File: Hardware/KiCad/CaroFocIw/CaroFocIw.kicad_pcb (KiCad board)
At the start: 4 copper layers, 92 x 42 mm, 105 parts, among them J1 Conn_01x04, J10 Conn_01x03, J11 Conn_01x03, J12 Conn_01x03, J13 Conn_01x03, J14 Conn_01x03, J15 Conn_01x04, J16 Conn_01x04, J17 Conn_01x04, J18 Conn_01x04, J19 Conn_01x04, J2 Conn_01x01, J20 Conn_01x04, J21 Conn_01x02, J22 Conn_01x02, J23 Conn_01x04, J3 Conn_01x01, J4 Conn_01x01, J7 Conn_01x02, J8 Conn_01x02, J9 Conn_01x03, Q1 Q_NMOS_SGD, Q2 Q_NMOS_SGD, Q3 Q_NMOS_SGD, Q4 Q_NMOS_SGD, Q5 Q_NMOS_SGD, Q6 Q_NMOS_SGD, U1 TCAN332, U2 STM32F405RGTx, U3 TLE7185-1E, U4 ACS711xEXLT-15AB, U5 AS5048A, U6 ACS711xEXLT-15AB, U7 ACS711xEXLT-15AB, U8 LMR16006YQ3

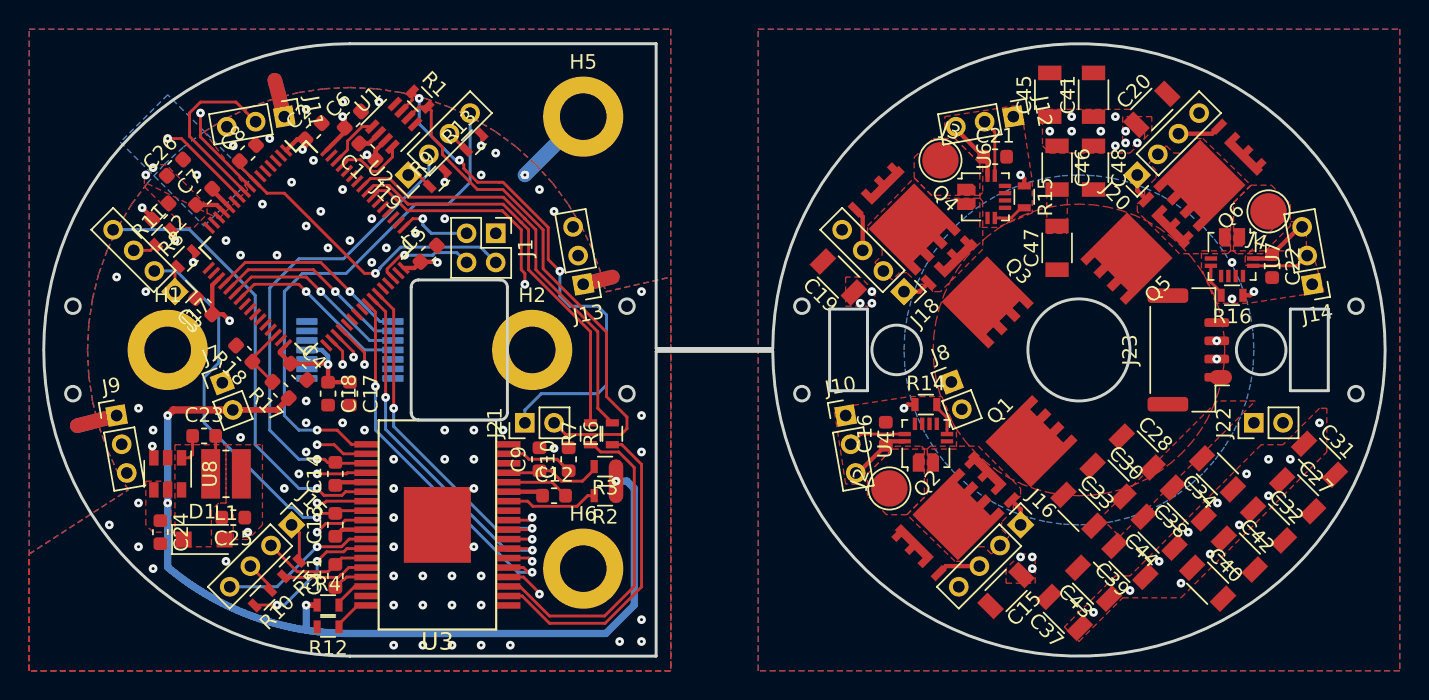
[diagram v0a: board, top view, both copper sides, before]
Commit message: some panelizing
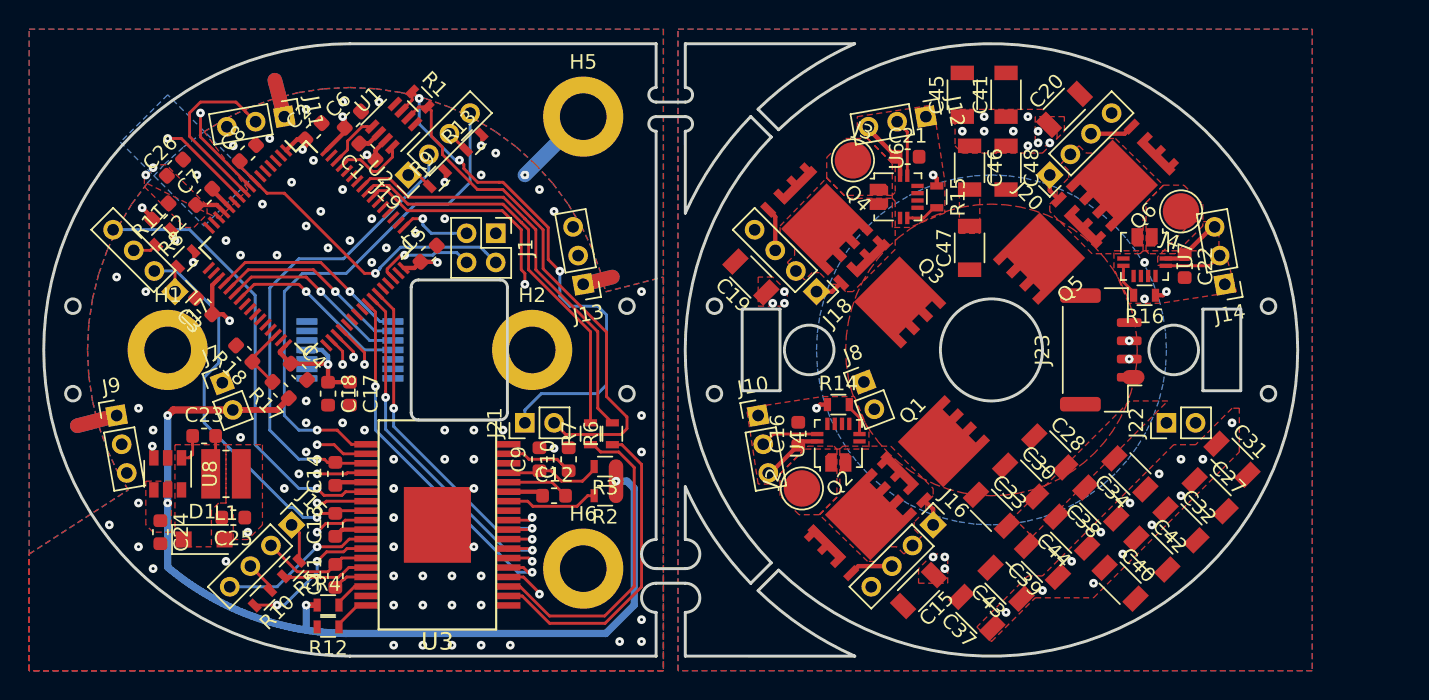
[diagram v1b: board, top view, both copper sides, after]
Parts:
- moved C15 6.00 mm to (199.0, 51.5)
- moved C16 6.00 mm to (190.8, 40.8)
- moved C19 6.00 mm to (187.5, 30.0)
- moved C20 6.00 mm to (209.0, 18.5)
- moved C21 6.00 mm to (198.2, 21.8)
- moved C22 6.00 mm to (217.2, 29.2)
- moved C27 6.00 mm to (219.0, 45.0)
- moved C28 6.00 mm to (208.0, 42.0)
- moved C30 6.00 mm to (206.0, 44.0)
- moved C31 6.00 mm to (220.5, 42.5)
- moved C32 6.00 mm to (217.0, 47.0)
- moved C33 6.00 mm to (204.0, 46.0)
- moved C34 6.00 mm to (213.5, 43.5)
- moved C37 6.00 mm to (203.0, 53.0)
- moved C38 6.00 mm to (211.5, 45.5)
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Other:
- board size 92 x 42 mm -> 86 x 42 mm

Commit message: preliminary version 1.0
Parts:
- removed the C31 at (220.5, 42.5)
- removed the C37 at (203.0, 53.0)
- removed the C41 at (205.0, 17.5)
- removed H5, H6: MountingHole_Pad, MountingHole:MountingHole_3.2mm_M3_ISO14580_Pad
- removed J21: Conn_01x02, Connector_PinHeader_2.00mm:PinHeader_1x02_P2.00mm_Vertical
- removed J23: Conn_01x04, Connector_JST:JST_GH_BM04B-GHS-TBT_1x04-1MP_P1.25mm_Vertical
- removed the J8 at (195.2, 37.2)
- removed the U1 at (163.0, 19.6)
- removed the U8 at (147.5, 43.5)
- added C29: 10µ 35V, Capacitor_SMD:C_1206_3216Metric, F.Cu at (46.0, 9.00)
- added C34: 10µ 35V, Capacitor_SMD:C_1206_3216Metric, F.Cu at (43.0, 18.0)
- added C38: 10µ 35V, Capacitor_SMD:C_1206_3216Metric, F.Cu at (45.0, -17.5)
- added G***: LOGO, libs:CDLC-Logo, B.Cu at (53.0, 16.0)
- added H3: MountingHole_Pad, MountingHole:MountingHole_3.2mm_M3_ISO14580_Pad, F.Cu at (16.0, -16.0)
- added H4: MountingHole_Pad, MountingHole:MountingHole_3.2mm_M3_ISO14580_Pad, F.Cu at (16.0, 16.0)
- added J2: Conn_01x01, TestPoint:TestPoint_Pad_D2.5mm, F.Cu at (34.5, -13.0)
- added J5: Conn_01x02, Connector_PinHeader_2.00mm:PinHeader_1x02_P2.00mm_Vertical, F.Cu at (-8.75, 2.25)
- added J6: Conn_01x02, Connector_PinHeader_2.00mm:PinHeader_1x02_P2.00mm_Vertical, F.Cu at (35.2, 2.25)
- added NT1: Net-Tie_2, NetTie:NetTie-2_SMD_Pad0.5mm, B.Cu at (-8.25, -10.2)
- added REF**: OSHW-Logo2_7.3x6mm_SilkScreen, Symbol:OSHW-Logo2_7.3x6mm_SilkScreen, B.Cu at (51.0, 4.00)
- added U5: ACS711xEXLT-15AB, Sensor_Current:Allegro_QFN-12-10-1EP_3x3mm_P0.5mm, F.Cu at (33.5, 6.50)
- added U9: LMR16006YQ3, Package_TO_SOT_SMD:SOT-23-6, F.Cu at (-12.5, 8.50)
- C10: value 2,2µ -> 4.7µ 25V
- C11, C12, C13, C14: value 1µ -> 4.7µ 25V
- C15, C19, C20: value 22μ, 25V -> 10μ 35V; footprint Capacitors_SMD:C_1206 -> Capacitor_SMD:C_1206_3216Metric
- C18, C25, C26: value 10μ -> 10μ 6.3V
- C2, C3, C4, C5, C6: value 2.2μ -> 4.7µ, 6.3V
- C24: value 10μ -> 10μ 35V
- C27, C28, C30: value C -> 10µ 35V; footprint Capacitors_SMD:C_1206 -> Capacitor_SMD:C_1206_3216Metric
- C31: renamed from C32; value C -> 10µ 35V; footprint Capacitors_SMD:C_1206 -> Capacitor_SMD:C_1206_3216Metric
- C32: renamed from C33; value C -> 10µ 35V; footprint Capacitors_SMD:C_1206 -> Capacitor_SMD:C_1206_3216Metric
- C33: renamed from C34; value C -> 10µ 35V; footprint Capacitors_SMD:C_1206 -> Capacitor_SMD:C_1206_3216Metric
- C35: renamed from C38; value C -> 10µ 35V; footprint Capacitors_SMD:C_1206 -> Capacitor_SMD:C_1206_3216Metric
- C36: renamed from C39; value C -> 10µ 35V; footprint Capacitors_SMD:C_1206 -> Capacitor_SMD:C_1206_3216Metric
- C37: renamed from C40; value C -> 10µ 35V; footprint Capacitors_SMD:C_1206 -> Capacitor_SMD:C_1206_3216Metric
- C39: renamed from C42; value C -> 10µ 35V; footprint Capacitors_SMD:C_1206 -> Capacitor_SMD:C_1206_3216Metric
- C40: renamed from C43; value C -> 10µ 35V; footprint Capacitors_SMD:C_1206 -> Capacitor_SMD:C_1206_3216Metric
- C41: renamed from C44; value C -> 10µ 35V; footprint Capacitors_SMD:C_1206 -> Capacitor_SMD:C_1206_3216Metric
- C42: renamed from C45; value C -> 10µ 35V; footprint Capacitors_SMD:C_1206 -> Capacitor_SMD:C_1206_3216Metric
- C43: renamed from C46; value C -> 10µ 35V; footprint Capacitors_SMD:C_1206 -> Capacitor_SMD:C_1206_3216Metric
- C44: renamed from C47; value C -> 10µ 35V; footprint Capacitors_SMD:C_1206 -> Capacitor_SMD:C_1206_3216Metric
- C45: renamed from C48; value C -> 10µ 35V; footprint Capacitors_SMD:C_1206 -> Capacitor_SMD:C_1206_3216Metric
- C7: value 10μ -> 4.7µ, 6.3V
- C9: value 2,2µ -> 4.7µ 35V
- D1: footprint Diodes_SMD:D_SOD-123F -> Diode_SMD:D_SOD-123F
- J13: value Conn_01x03 -> Conn_01x04; footprint Connector_PinHeader_2.00mm:PinHeader_1x03_P2.00mm_Vertical -> Connector_PinHeader_2.00mm:PinHeader_1x04_P2.00mm_Vertical
- J19: value Conn_01x04 -> Conn_01x02; footprint Connector_PinHeader_2.00mm:PinHeader_1x04_P2.00mm_Vertical -> Connector_PinHeader_2.00mm:PinHeader_1x02_P2.00mm_Vertical
- J4: value Conn_01x01 -> Conn_01x04_MountingPin; footprint TestPoint:TestPoint_Pad_D2.5mm -> Connector_JST:JST_GH_BM04B-GHS-TBT_1x04-1MP_P1.25mm_Vertical
- J7: value Conn_01x02 -> Conn_01x03; footprint Connector_PinHeader_2.00mm:PinHeader_1x02_P2.00mm_Vertical -> Connector_PinHeader_2.00mm:PinHeader_1x03_P2.00mm_Vertical
- L1: footprint Inductors_SMD:L_Wuerth_MAPI-3015 -> Inductor_SMD:L_Wuerth_MAPI-3015
- Q1, Q2, Q3, Q4, Q5, Q6: value Q_NMOS_SGD -> BSZ013NE2LS5I; footprint libs:TDSON-8_FL -> libs:PG-TSDSON-8-FL
- R1, R10, R11, R12, R13, R14, R15, R16, R2, R3, R4, R5, R8, R9: footprint Resistors_SMD:R_0603 -> Resistor_SMD:R_0603_1608Metric
- R6, R7: value 4.7k -> 10k; footprint Resistors_SMD:R_0603 -> Resistor_SMD:R_0603_1608Metric
- U2: value STM32F405RGTx -> TCAN332; footprint Package_QFP:LQFP-64_10x10mm_P0.5mm -> Package_TO_SOT_SMD:SOT-23-8
- U3: value TLE7185-1E -> STM32F405RGTx; footprint libs:PG-DSO-36-38 -> Package_QFP:LQFP-64_10x10mm_P0.5mm
- U4: value ACS711xEXLT-15AB -> TLE7185-1E; footprint Sensor_Current:Allegro_QFN-12-10-1EP_3x3mm_P0.5mm -> libs:PG-DSO-36-38
- moved U4 189.8 mm to (6.00, 12.0)
- moved J13 180.9 mm to (-4.00, 12.0), turned to 315 degrees
- moved U3 177.4 mm to (-3.00, -7.00), turned to 315 degrees
- moved J15 175.6 mm to (-12.0, -4.00), turned to 225 degrees
- moved J7 170.4 mm to (-16.0, 4.50), turned to 10 degrees
- moved J4 167.5 mm to (51.5, 0.00), turned to 90 degrees
- moved Q3 165.0 mm to (36.0, -5.00), turned to 135 degrees
- moved Q1 164.6 mm to (39.0, 8.00), turned to 225 degrees
- moved Q4 164.0 mm to (31.8, -9.21), turned to 135 degrees
- moved Q2 163.9 mm to (34.8, 12.2), turned to 225 degrees
- moved C19 163.8 mm to (27.5, -5.30)
- moved C1 163.8 mm to (1.20, -13.6)
- moved C10 163.8 mm to (15.0, 7.50)
- moved C11 163.8 mm to (-1.00, 15.5)
- moved C12 163.8 mm to (14.0, 10.0)
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- renumbered J12 to J10, J14 to J12, J16 to J14, J18 to J16, J20 to J18, J22 to J20, J10 to J8, J2 to U1, U5 to U6, U6 to U7, U7 to U8
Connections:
- J11 pad 2: /MCU/CurrentV -> /MCU/CurrentW
- J13 pad 1: GNDA -> /GateDriver/GateUH
- J13 pad 2: /MCU/CurrentW -> /GateDriver/SourceUH
- J13 pad 3: +3.3VA -> /GateDriver/GateUL
- J15 pad 1: /GateDriver/GateUH -> /GateDriver/GateVH
- J15 pad 2: /GateDriver/SourceUH -> /GateDriver/SourceVH
- J15 pad 3: /GateDriver/GateUL -> /GateDriver/GateVL
- J15 pad 4: /GateDriver/SourceUL -> /GateDriver/SourceVL
- J17 pad 1: /GateDriver/GateVH -> /GateDriver/GateWH
- J17 pad 2: /GateDriver/SourceVH -> /GateDriver/SourceWH
- J17 pad 3: /GateDriver/GateVL -> /GateDriver/GateWL
- J17 pad 4: /GateDriver/SourceVL -> /GateDriver/SourceWL
- J19 pad 1: /GateDriver/GateWH -> /Can/CanH
- J19 pad 2: /GateDriver/SourceWH -> /Can/CanL
- J3 pad 1: /CurrentSensingV/PhaseOut -> /CurrentsensingW/PhaseOut
- J4 pad 1: /CurrentsensingW/PhaseOut -> GNDPWR
- J7 pad 1: GND -> GNDA
- J7 pad 2: BattA -> /MCU/CurrentU
- J9 pad 2: /MCU/CurrentU -> /MCU/CurrentV
- U2 pad 1: +3V3 -> /Can/CanTx
- U2 pad 2: (no net) -> GND
- U2 pad 3: (no net) -> +3V3
- U2 pad 4: (no net) -> /Can/CanRx
- U2 pad 6: (no net) -> /Can/CanL
- U2 pad 7: /MCU/~RST -> /Can/CanH
- U2 pad 8: /MCU/CurrentW -> (no net)
- U3 pad 1: (no net) -> +3V3
- U3 pad 10: /GateDriver/LogicWL -> /MCU/CurrentU
- U3 pad 11: GND -> (no net)
- U3 pad 12: Net-(R2-Pad2) -> GNDA
- U3 pad 13: Net-(C12-Pad1) -> +3.3VA
- U3 pad 14: Net-(C12-Pad2) -> (no net)
- U3 pad 15: Net-(C9-Pad1) -> (no net)
- U3 pad 16: GND -> (no net)
- U3 pad 17: Net-(C10-Pad1) -> (no net)
- U3 pad 19: /GateDriver/SourceWL -> +3V3
- U3 pad 2: Net-(R6-Pad1) -> (no net)
- U3 pad 20: /GateDriver/Gate_W_L_bR -> /Encoder/~EncoderCs
- U3 pad 21: /GateDriver/SourceWH -> /Encoder/EncoderSclk
- U3 pad 22: /GateDriver/GateWHbR -> /Encoder/EncoderMiso
- U3 pad 23: Net-(C14-Pad1) -> /Encoder/EncoderMosi
- U3 pad 24: /GateDriver/SourceVL -> (no net)
- U3 pad 25: /GateDriver/Gate_V_L_bR -> (no net)
- U3 pad 26: /GateDriver/SourceVH -> (no net)
- U3 pad 27: /GateDriver/GateVHbR -> (no net)
- U3 pad 28: Net-(C13-Pad1) -> (no net)
- U3 pad 29: /GateDriver/SourceUL -> (no net)
- U3 pad 3: Net-(R7-Pad1) -> (no net)
- U3 pad 30: /GateDriver/Gate_U_L_bR -> /DcLinkVoltageSensing/AnalogOut
- U3 pad 31: /GateDriver/SourceUH -> (no net)
- U3 pad 32: /GateDriver/GateUHbR -> +3V3
- U3 pad 33: Net-(C11-Pad1) -> (no net)
- U3 pad 34: Net-(R4-Pad2) -> /GateDriver/LogicUL
- U3 pad 35: GND -> /GateDriver/LogicVL
- U3 pad 36: Net-(R12-Pad1) -> /GateDriver/LogicWL
- U3 pad 37: GND -> (no net)
- U3 pad 4: /MCU/GateDriverEnable -> (no net)
- U3 pad 5: /MCU/LogicUH -> (no net)
- U3 pad 6: /GateDriver/LogicUL -> (no net)
- U3 pad 7: /MCU/LogicVH -> /MCU/~RST
- U3 pad 8: /GateDriver/LogicVL -> /MCU/CurrentW
- U3 pad 9: /MCU/LogicWH -> /MCU/CurrentV
- U4 pad 1: /CurrentSensingU/PhaseOut -> (no net)
- U4 pad 10: 3.3VA_U -> /GateDriver/LogicWL
- U4 pad 2: /CurrentSensingU/PhaseIn -> Net-(R6-Pad1)
- U4 pad 3: AGND_U -> Net-(R7-Pad1)
- U4 pad 4: Net-(R14-Pad2) -> /MCU/GateDriverEnable
- U4 pad 5: AGND_U -> /MCU/LogicUH
- U4 pad 6: AGND_U -> /GateDriver/LogicUL
- U4 pad 7: AGND_U -> /MCU/LogicVH
- U4 pad 8: AGND_U -> /GateDriver/LogicVL
- U4 pad 9: /CurrentSensingU/AnalogOut -> /MCU/LogicWH
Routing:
- net GNDA: track 24.1 -> 16.8 mm, vias 1 -> 38
- net /GateDriver/LogicWL: track 22.9 -> 25.4 mm
- net /MCU/GateDriverEnable: track 50.5 -> 52.7 mm
- net /Can/CanH: track 36.8 -> 38.5 mm
- net /GateDriver/SourceWL: track 35.5 -> 36.7 mm
- net /Can/CanL: track 35.9 -> 37.0 mm
- net GNDPWR: track 0.55 -> 1.50 mm, vias 0 -> 51
- net /MCU/SWDIO: track 7.01 -> 7.91 mm
- net /HalfBridgeU/GateH: track 1.95 -> 2.84 mm
- net /HalfBridgeV/GateH: track 1.95 -> 2.84 mm
- net /HalfBridgeW/GateH: track 1.95 -> 2.84 mm
- net +3V3: track 25.4 -> 26.2 mm
- net Net-(R6-Pad1): track 21.9 -> 22.6 mm
- net /GateDriver/Gate_W_L_bR: track 34.7 -> 35.4 mm
- net GND: track 7.29 -> 7.50 mm, vias 74 -> 83
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- added copper zone on B.Cu, net (none)
- added copper zone on F.Cu, net (none)
- added copper zone on In1.Cu, net (none)
- added copper zone on In2.Cu, net (none)
- added copper zone on In2.Cu, net +3.3VA
- added copper zone on In1.Cu, net GNDA
- removed copper zone on In1.Cu, net +3.3VA
- removed copper zone on In2.Cu, net GNDA
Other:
- board size 86 x 42 mm -> 85 x 42 mm
- board text added: "09/2019"
- board text added: "3V3A"
- board text added: "AGND"
- board text added: "Batt"
- board text added: "CanH"
- board text added: "CanL"
- board text added: "CaroFocIW Version 1.0"
- board text added: "CrrntSns"
- board text added: "GND"
- board text added: "GateH"
- board text added: "GateL"
- board text added: "JLCJLCJLCJLC"
- board text added: "SWCLK"
- board text added: "SWDIO"
- board text added: "SourceH"
- board text added: "SourceL"
- board text added: "Supply+"
- board text added: "Supply-"
- board text added: "U"
- board text added: "V"
- board text added: "W"
- board text added: "designed by O. H. Maier 09/2019"
- board text added: "~RST"
